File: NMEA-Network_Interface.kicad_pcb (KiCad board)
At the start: 4 copper layers, 135 x 56 mm, 59 parts, among them J1 Conn_01x02, J2 USB_C_Receptacle_USB2.0_16P, J3 Conn_01x04, J4 Raspberry_Pi_4, J6 Conn_Coaxial_Small, J7 Conn_Coaxial_Small, Q1 MMBT3904, Q2 MMBT3904, Q3 MMBT3904, Q4 MMBT3904, U1 ESP32-WROOM-32E, U2 AG9905-LP, U3 dAISy-catcher, U4 HY931147C, U5 LAN8720A, U7 SMN-304, U8 SIM7080G

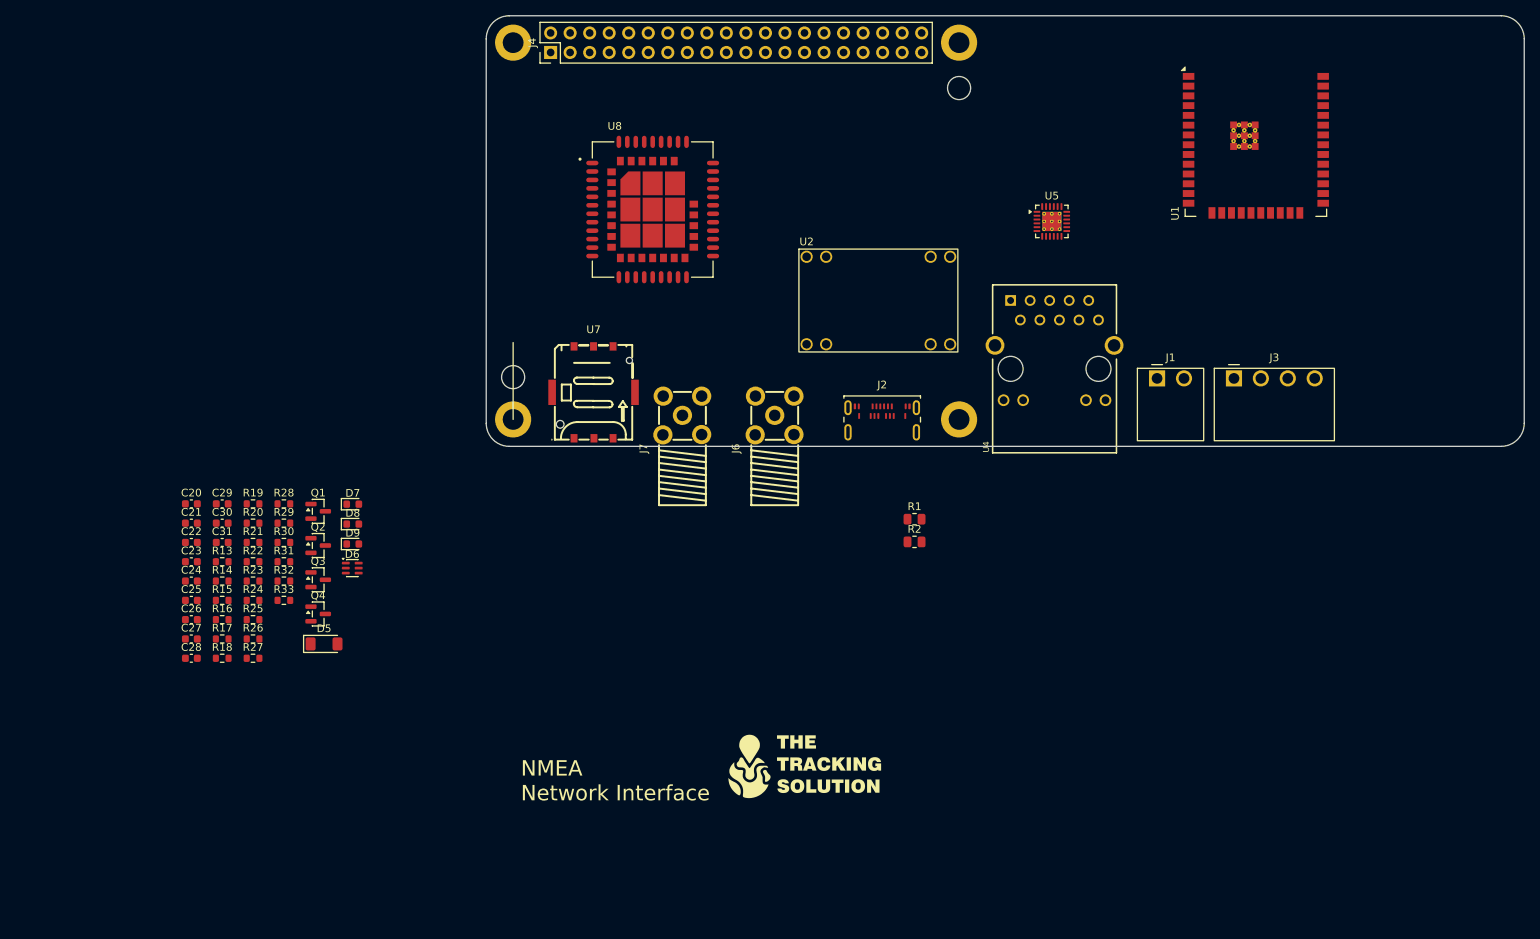
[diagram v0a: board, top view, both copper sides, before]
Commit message: Adding ethernet module and more
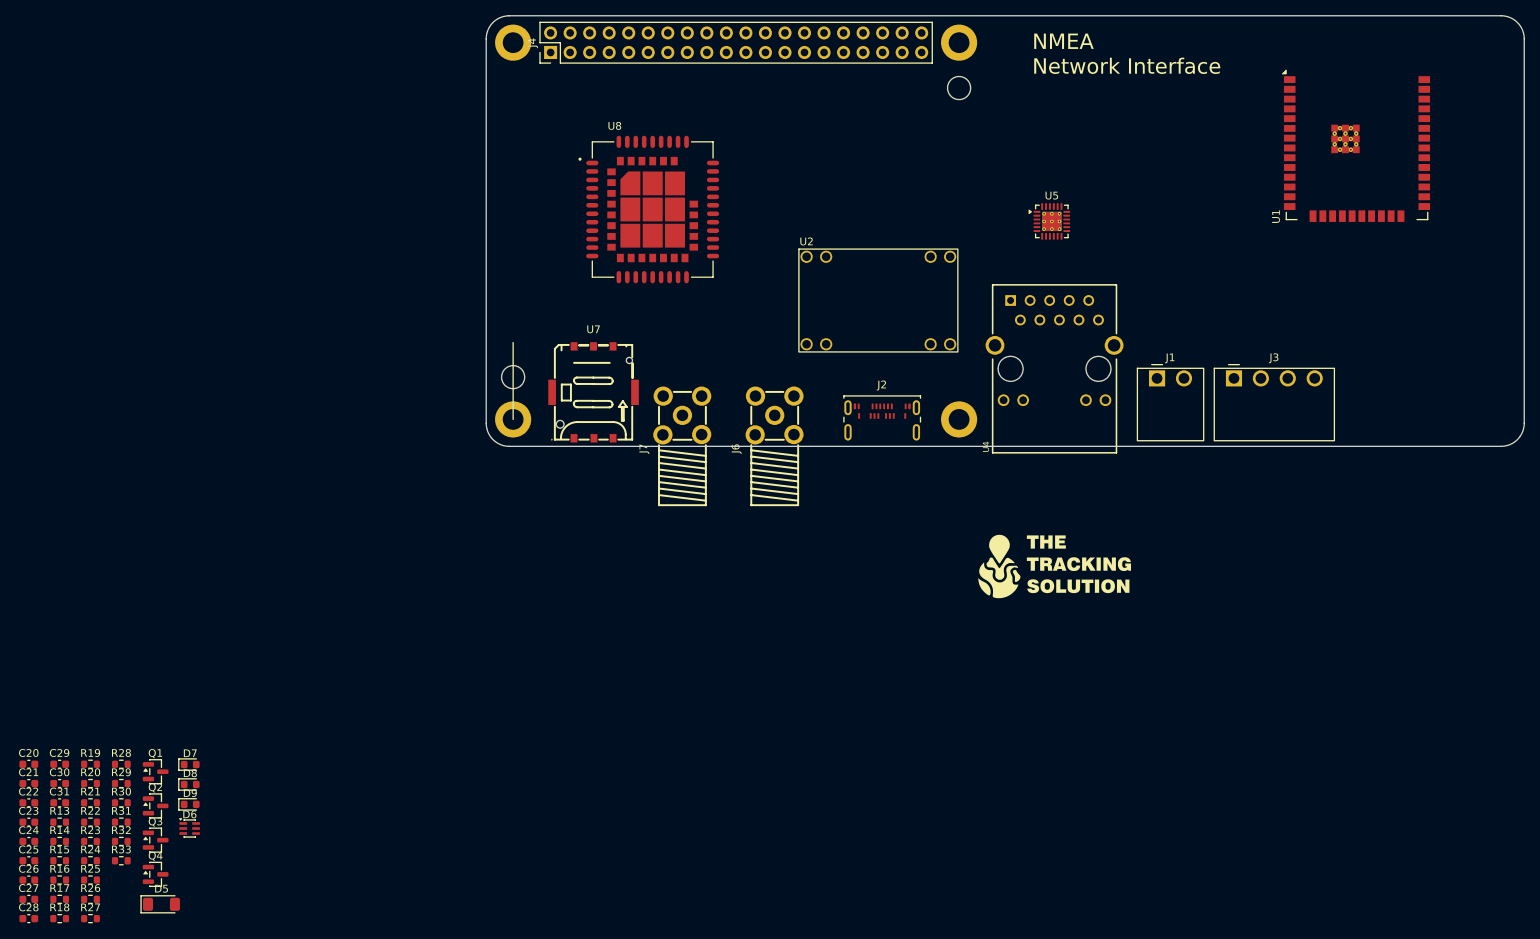
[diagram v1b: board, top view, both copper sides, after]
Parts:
- removed R1, R2: 5k1, Resistor_SMD:R_0805_2012Metric
- U3: value dAISy-catcher -> New Version
- moved G*** 41.6 mm to (190.5, 139.0)
- moved C29 39.9 mm to (61.0, 164.8)
- moved C31 39.9 mm to (61.0, 169.9)
- moved R13 39.9 mm to (61.0, 172.4)
- moved R15 39.9 mm to (61.0, 177.4)
- moved R16 39.9 mm to (61.0, 179.9)
- moved R18 39.9 mm to (61.0, 184.9)
- moved C20 39.9 mm to (57.0, 164.8)
- moved C22 39.9 mm to (57.0, 169.9)
- moved C23 39.9 mm to (57.0, 172.4)
- moved C25 39.9 mm to (57.0, 177.4)
- moved C26 39.9 mm to (57.0, 179.9)
- moved C28 39.9 mm to (57.0, 184.9)
- moved D5 39.9 mm to (74.3, 183.1)
- moved D9 39.9 mm to (78.0, 170.1)
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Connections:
- net /Power/VP_USB renamed Net-(J2-VBUS-PadA4)
- J2 pad A1: GND -> Net-(J2-GND-PadA1)
- J2 pad A12: GND -> Net-(J2-GND-PadA1)
- J2 pad A5: Net-(J2-CC1) -> unconnected-(J2-CC1-PadA5)
- J2 pad A6: Net-(J2-D+-PadA6) -> unconnected-(J2-D+-PadA6)
- J2 pad A7: Net-(J2-D--PadA7) -> unconnected-(J2-D--PadA7)
- J2 pad B1: GND -> Net-(J2-GND-PadA1)
- J2 pad B12: GND -> Net-(J2-GND-PadA1)
- J2 pad B5: Net-(J2-CC2) -> unconnected-(J2-CC2-PadB5)
- J2 pad B6: Net-(J2-D+-PadA6) -> unconnected-(J2-D+-PadB6)
- J2 pad B7: Net-(J2-D--PadA7) -> unconnected-(J2-D--PadB7)
- U4 pad V+: /Power/VP_PoE -> unconnected-(U4-PadV+)
- U4 pad V-: /Power/VN_PoE -> unconnected-(U4-PadV-)
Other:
- copper layers 4 -> 2
- board text removed: "NMEA2000"
